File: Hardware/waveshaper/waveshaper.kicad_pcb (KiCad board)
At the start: 2 copper layers, 57 x 154 mm, 47 parts, among them J12 1x3 pin socket, J13 EURO_PWR_2x5, J14 1x6 pin socket, J15 1x6 pin socket, J25 3 pin Molex header, J27 3 pin Molex header, J29 3 pin Molex header, J30 2x5 pin socket, J32 3 pin Molex header, J34 3 pin Molex header, J36 3 pin Molex header, J38 3 pin Molex header, SW1 SW_SPDT, U4 4066, U5 4066

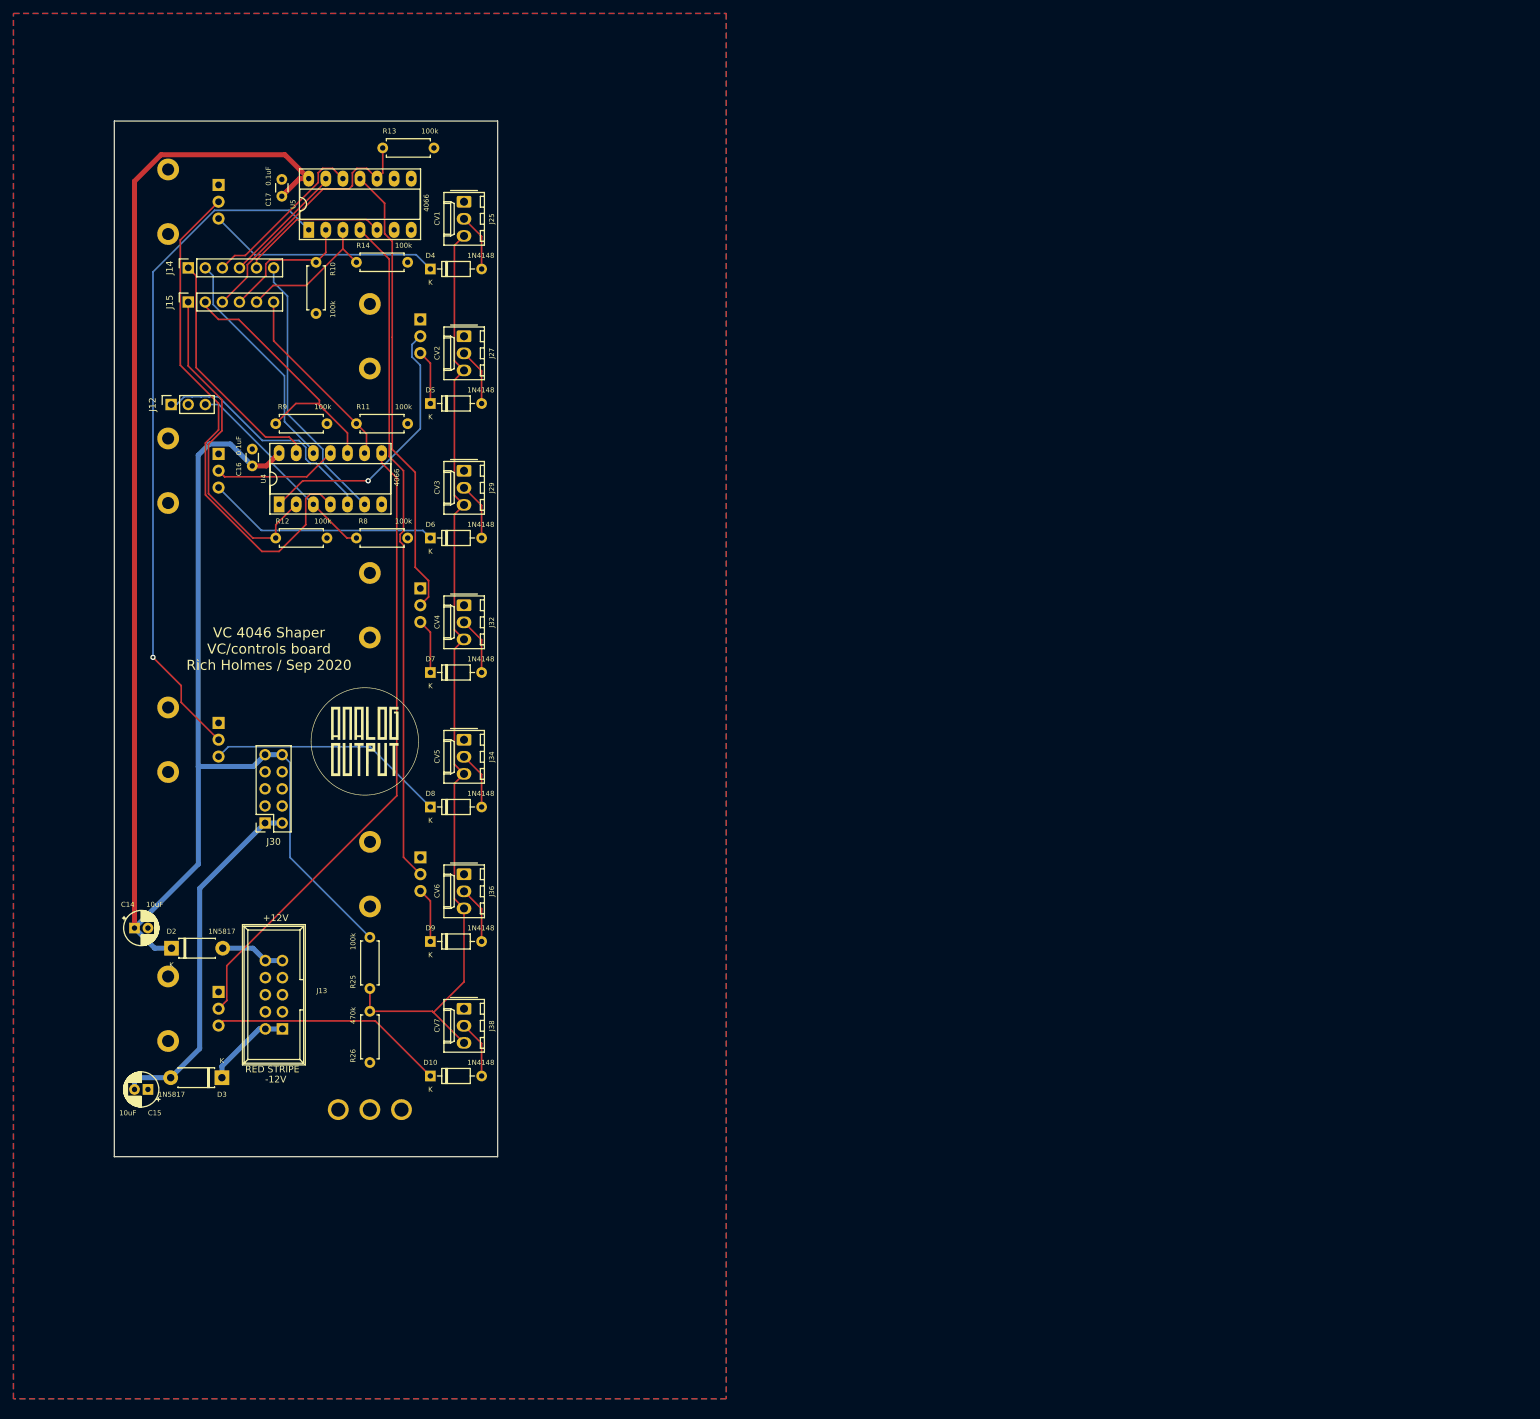
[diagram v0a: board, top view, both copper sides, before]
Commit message: Overdue commit: Boards redesign, docs folder
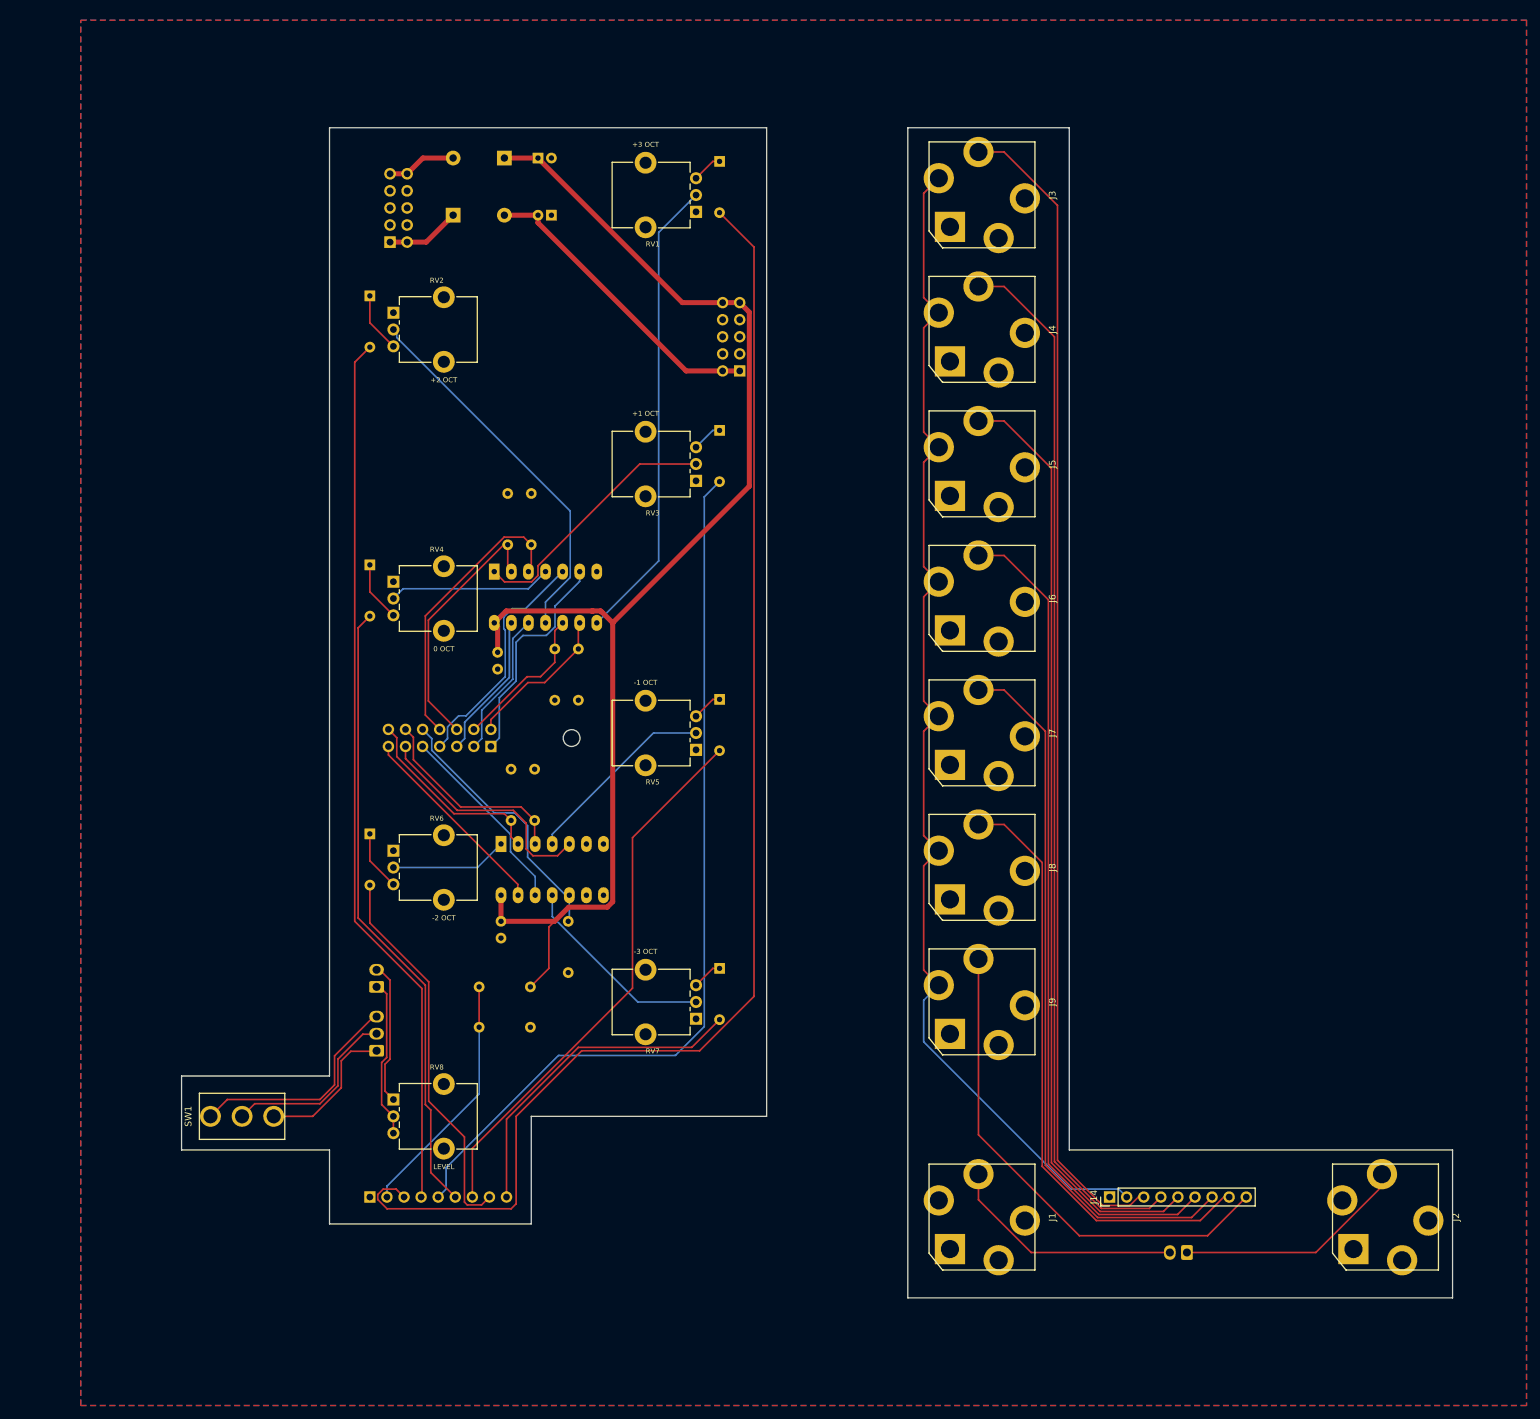
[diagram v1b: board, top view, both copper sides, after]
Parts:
- removed the G*** at (119.2, 110.2)
- removed the G*** at (120.0, 105.0)
- removed J25, J27, J29, J32, J34, J36, J38: 3 pin Molex header, ao_tht:Molex_KK-254_AE-6410-03A_1x03_P2.54mm_Vertical
- added G***: LOGO, ao_tht:analogoutput, B.Cu at (210.5, 165.2)
- added G***: LOGO, ao_tht:analogoutput, B.Cu at (128.2, 68.0)
- added J1: AudioJack2_SwitchT, ao_tht:Jack_6.35mm_PJ_629HAN, F.Cu at (211.0, 181.0)
- added J10: 2x7 IDC header, Connector_PinHeader_2.54mm:PinHeader_2x07_P2.54mm_Vertical, B.Cu at (138.0, 111.0)
- added J11: Conn_01x03, ao_tht:Molex_KK-254_AE-6410-03A_1x03_P2.54mm_Vertical, B.Cu at (121.0, 156.2)
- added J2: AudioJack2_SwitchT, ao_tht:Jack_6.35mm_PJ_629HAN, F.Cu at (271.0, 181.0)
- added J20: Conn_01x02, ao_tht:Molex_KK-254_AE-6410-02A_1x02_P2.54mm_Vertical, B.Cu at (121.0, 146.8)
- added J3: AudioJack2_SwitchT, ao_tht:Jack_6.35mm_PJ_629HAN, F.Cu at (211.0, 29.0)
- added J4: AudioJack2_SwitchT, ao_tht:Jack_6.35mm_PJ_629HAN, F.Cu at (211.0, 49.0)
- added J5: AudioJack2_SwitchT, ao_tht:Jack_6.35mm_PJ_629HAN, F.Cu at (211.0, 69.0)
- added J6: AudioJack2_SwitchT, ao_tht:Jack_6.35mm_PJ_629HAN, F.Cu at (211.0, 89.0)
- added J7: AudioJack2_SwitchT, ao_tht:Jack_6.35mm_PJ_629HAN, F.Cu at (211.0, 109.0)
- added J8: AudioJack2_SwitchT, ao_tht:Jack_6.35mm_PJ_629HAN, F.Cu at (211.0, 129.0)
- added J9: AudioJack2_SwitchT, ao_tht:Jack_6.35mm_PJ_629HAN, F.Cu at (211.0, 149.0)
- added REF**: MountingHole_2.5mm, MountingHole:MountingHole_2.5mm, F.Cu at (150.0, 109.8)
- added RV8: A100k, ao_tht:Potentiometer_Alpha_RD901F-40-00D_Single_Vertical_CircularHoles_centered, F.Cu at (131.0, 166.0)
- C14, C15, C16, C17, D10, D2, D3, D4, D5, D6, D7, D8, D9, G***, J13, J30, R10, R11, R12, R13, R14, R25, R26, R8, R9, U4, U5: moved to B.Cu
- J12: value 1x3 pin socket -> Conn_01x02; footprint Connector_PinSocket_2.54mm:PinSocket_1x03_P2.54mm_Vertical -> ao_tht:Molex_KK-254_AE-6410-02A_1x02_P2.54mm_Vertical; moved to B.Cu
- J14: value 1x6 pin socket -> Conn_01x9; footprint Connector_PinSocket_2.54mm:PinSocket_1x06_P2.54mm_Vertical -> Connector_PinHeader_2.54mm:PinHeader_1x09_P2.54mm_Vertical
- J15: value 1x6 pin socket -> Conn_01x9; footprint Connector_PinSocket_2.54mm:PinSocket_1x06_P2.54mm_Vertical -> Connector_PinSocket_2.54mm:PinSocket_1x09_P2.54mm_Vertical; moved to B.Cu
- RV1, RV2, RV3, RV4, RV5, RV6, RV7: footprint ao_tht:Potentiometer_Alpha_RD901F-40-00D_Single_Vertical_CircularHoles -> ao_tht:Potentiometer_Alpha_RD901F-40-00D_Single_Vertical_CircularHoles_centered; moved to F.Cu
- SW1: moved to F.Cu
- moved J12 196.8 mm to (241.5, 186.2), turned to 180 degrees
- moved J14 194.6 mm to (230.0, 178.0)
- moved C15 143.2 mm to (147.0, 32.0)
- moved J15 135.8 mm to (120.0, 178.0), turned to 270 degrees
- moved D3 132.8 mm to (132.4, 32.0), turned to 0 degrees
- moved C14 129.3 mm to (145.0, 23.5)
- moved D2 127.5 mm to (140.0, 23.5), turned to 180 degrees
- moved J13 118.1 mm to (123.0, 36.0), turned to 0 degrees
- moved C17 112.6 mm to (139.5, 137.0), turned to 270 degrees
- moved J30 97.5 mm to (175.0, 55.2), turned to 0 degrees
- moved R10 89.1 mm to (144.5, 122.0), turned to 90 degrees
- moved R14 86.1 mm to (141.0, 122.0), turned to 90 degrees
- moved R11 80.4 mm to (149.5, 137.0), turned to 270 degrees
- moved G*** 68.2 mm to (160.0, 86.8)
- moved RV1 63.5 mm to (161.0, 29.0)
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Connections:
- J12 pad 1: Net-(J12-Pad1) -> /Panel and power/OUT
- J12 pad 2: Net-(J12-Pad2) -> /Panel and power/IN
- J14 pad 1: Net-(J14-Pad1) -> GND
- J14 pad 3: Net-(J14-Pad3) -> /Panel and power/CVIN_+3
- J14 pad 4: Net-(J14-Pad4) -> /Panel and power/CVIN_+2
- J14 pad 5: Net-(J14-Pad5) -> /Panel and power/CVIN_+1
- J14 pad 6: Net-(J14-Pad6) -> /Panel and power/CVIN_0
- J15 pad 1: Net-(J15-Pad1) -> GND
- J15 pad 2: Net-(J15-Pad2) -> +10V
- J15 pad 3: Net-(J15-Pad3) -> Net-(D4-Pad2)
- J15 pad 4: Net-(J15-Pad4) -> Net-(D5-Pad2)
- J15 pad 5: Net-(J15-Pad5) -> Net-(D6-Pad2)
- J15 pad 6: Net-(J15-Pad6) -> Net-(D7-Pad2)
- R10 pad 1: Net-(J15-Pad4) -> MIXIN_-1
- R11 pad 1: Net-(J15-Pad6) -> MIXIN_-3
- R12 pad 1: Net-(J15-Pad1) -> MIXIN_+2
- R13 pad 1: Net-(J15-Pad3) -> MIXIN_0
- R14 pad 1: Net-(J15-Pad5) -> MIXIN_-2
- R8 pad 1: Net-(J12-Pad3) -> MIXIN_+3
- R9 pad 1: Net-(J15-Pad2) -> MIXIN_+1
- SW1 pad 1: Net-(J17-Pad1) -> /Panel and power/SL_MED
- SW1 pad 2: Net-(J23-Pad1) -> /Panel and power/SLEW
- SW1 pad 3: Net-(J18-Pad1) -> /Panel and power/SL_HIGH
- U4 pad 1: CV_+2 -> CV_-2
- U4 pad 10: Net-(J15-Pad2) -> MIXIN_-3
- U4 pad 11: CV_+1 -> CV_-3
- U4 pad 12: Net-(J14-Pad2) -> /RIPOUT_-3
- U4 pad 13: Net-(J14-Pad1) -> /RIPOUT_-2
- U4 pad 2: Net-(J15-Pad1) -> MIXIN_-2
- U4 pad 3: Net-(J12-Pad3) -> MIXIN_-1
- U4 pad 4: CV_+3 -> CV_-1
- U4 pad 5: Net-(J12-Pad1) -> /RIPOUT_-1
- U4 pad 6: Net-(J14-Pad6) -> GND
- U4 pad 8: CV_-3 -> GND
- U4 pad 9: Net-(J15-Pad6) -> GND
- U5 pad 1: CV_-1 -> CV_+1
- U5 pad 10: Net-(J15-Pad3) -> MIXIN_+2
- U5 pad 11: CV_0 -> CV_+2
- U5 pad 12: Net-(J14-Pad3) -> /RIPOUT_+2
- U5 pad 13: Net-(J14-Pad4) -> /RIPOUT_+1
- U5 pad 2: Net-(J15-Pad4) -> MIXIN_+1
- U5 pad 3: Net-(J15-Pad5) -> MIXIN_0
- U5 pad 4: CV_-2 -> CV_0
- U5 pad 5: Net-(J14-Pad5) -> /RIPOUT_0
- U5 pad 6: GND -> /RIPOUT_+3
- U5 pad 8: GND -> CV_+3
- U5 pad 9: GND -> MIXIN_+3
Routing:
- net Net-(D4-Pad2): track 8.55 -> 201.4 mm
- net /Panel and power/CVIN_+3: track 0.00 -> 173.2 mm
- net /Panel and power/CVIN_+2: track 0.00 -> 156.4 mm
- net Net-(J14-Pad2): track 34.2 -> 180.3 mm
- net /Panel and power/CVIN_+1: track 0.00 -> 139.7 mm
- net Net-(D6-Pad2): track 8.55 -> 133.9 mm
- net /Panel and power/CVIN_0: track 0.00 -> 123.0 mm
- net Net-(D5-Pad2): track 8.55 -> 131.5 mm
- net /Panel and power/CVIN_-1: track 0.00 -> 106.3 mm
- net +10V: track 142.6 -> 36.9 mm
- net /Panel and power/CVIN_-2: track 0.00 -> 89.6 mm
- net +12V: track 286.7 -> 198.7 mm
- net Net-(D7-Pad2): track 8.55 -> 93.1 mm
- net CV_-2: track 100.0 -> 17.4 mm
- net /Panel and power/CVIN_-3: track 0.00 -> 74.6 mm
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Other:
- board size 57 x 154 mm -> 189 x 174 mm
- board text added: "CCW"
- board text added: "HIGH"
- board text added: "IN"
- board text added: "MED"
- board text added: "OUT"
- board text added: "Rich Holmes Oct 2020"
- board text added: "SLEW"
- board text added: "Voltage Controlled 4046 Wave Shaper jack board"
- board text added: "Voltage Controlled 4046 Wave Shaper pot/switch board Rich Holmes Oct 2020"
- board text added: "WIPER"
- board text removed: "VC 4046 Shaper VC/controls board Rich Holmes / Sep 2020"
